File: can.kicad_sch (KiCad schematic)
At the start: 11 parts, among them U2 SN65HVD230

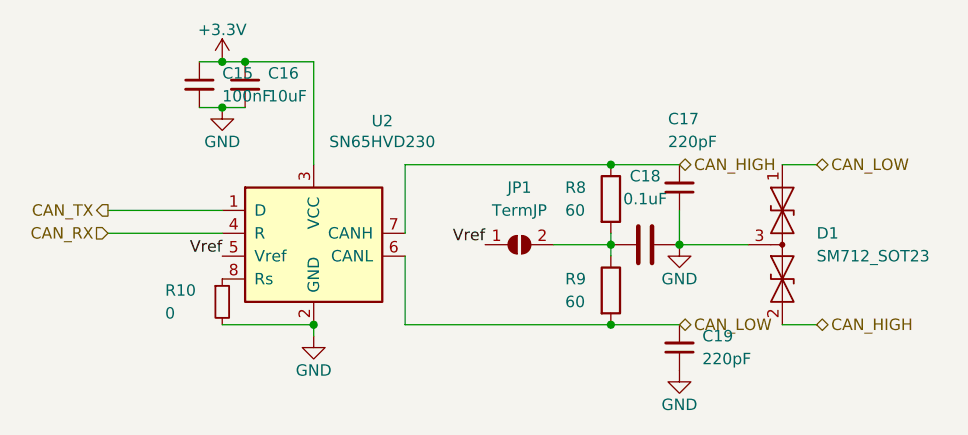
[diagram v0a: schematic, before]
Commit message: Some routing
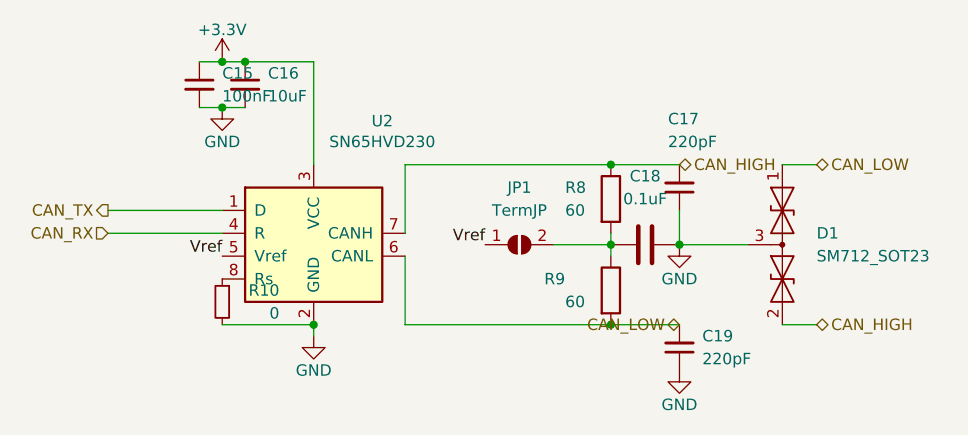
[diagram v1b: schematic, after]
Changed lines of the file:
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@@
     (effects (font (size 1.27 1.27)) (justify left))
   )
-  (hierarchical_label "CAN_LOW" (shape bidirectional) (at 175.26 97.79 0) (fields_autoplaced)
-    (effects (font (size 1.27 1.27)) (justify left))
+  (hierarchical_label "CAN_LOW" (shape bidirectional) (at 175.26 97.79 180) (fields_autoplaced)
+    (effects (font (size 1.27 1.27)) (justify right))
   )
   (symbol (lib_id "power:GND") (at 134.62 99.06 0) (unit 1)
@@
     )
   )
-  (symbol (lib_id "Device:R_Small") (at 124.46 95.25 0) (unit 1)
+  (symbol (lib_id "Device:R_Small") (at 124.46 95.25 0) (mirror y) (unit 1)
     (in_bom yes) (on_board yes) (dnp no)
-    (property "Reference" "R10" (at 118.11 93.98 0)
-      (effects (font (size 1.27 1.27)) (justify left))
-    )
-    (property "Value" "0" (at 118.11 96.52 0)
+    (property "Reference" "R10" (at 130.81 93.98 0)
+      (effects (font (size 1.27 1.27)) (justify left))
+    )
+    (property "Value" "0" (at 130.81 96.52 0)
       (effects (font (size 1.27 1.27)) (justify left))
     )
@@
   )
   (symbol (lib_id "Device:R") (at 167.64 93.98 0) (unit 1)
-    (in_bom yes) (on_board yes) (dnp no) (fields_autoplaced)
+    (in_bom yes) (on_board yes) (dnp no)
     (property "Reference" "R9" (at 162.56 92.71 0)
-      (effects (font (size 1.27 1.27)) (justify left))
+      (effects (font (size 1.27 1.27)) (justify right))
     )
     (property "Value" "60" (at 162.56 95.25 0)
